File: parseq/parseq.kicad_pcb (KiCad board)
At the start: 2 copper layers, 47.5 x 55 mm, 46 parts, among them J1 Conn_01x01, J2 Conn_01x01, J3 Conn_01x01, J4 Conn_01x01, U1 Opamp_Quad, U2 Opamp_Dual

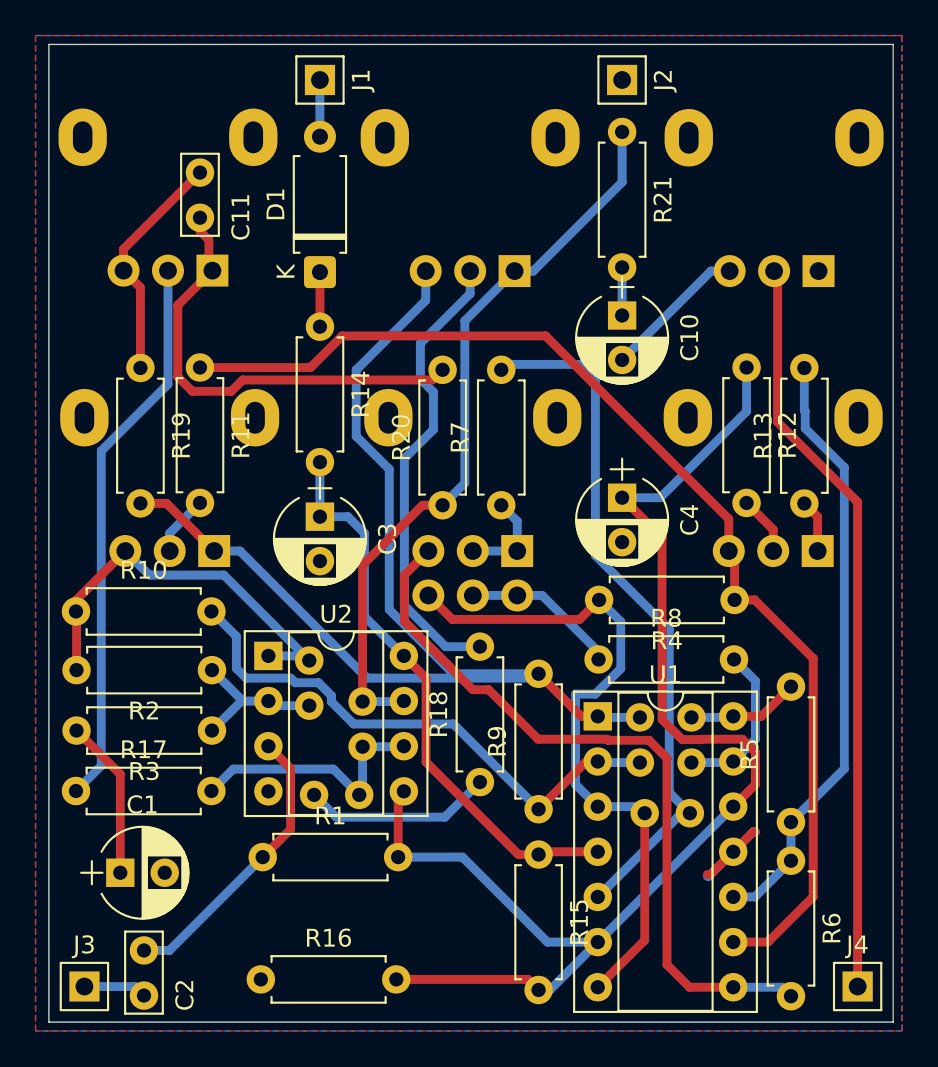
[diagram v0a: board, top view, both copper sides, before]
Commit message: update board
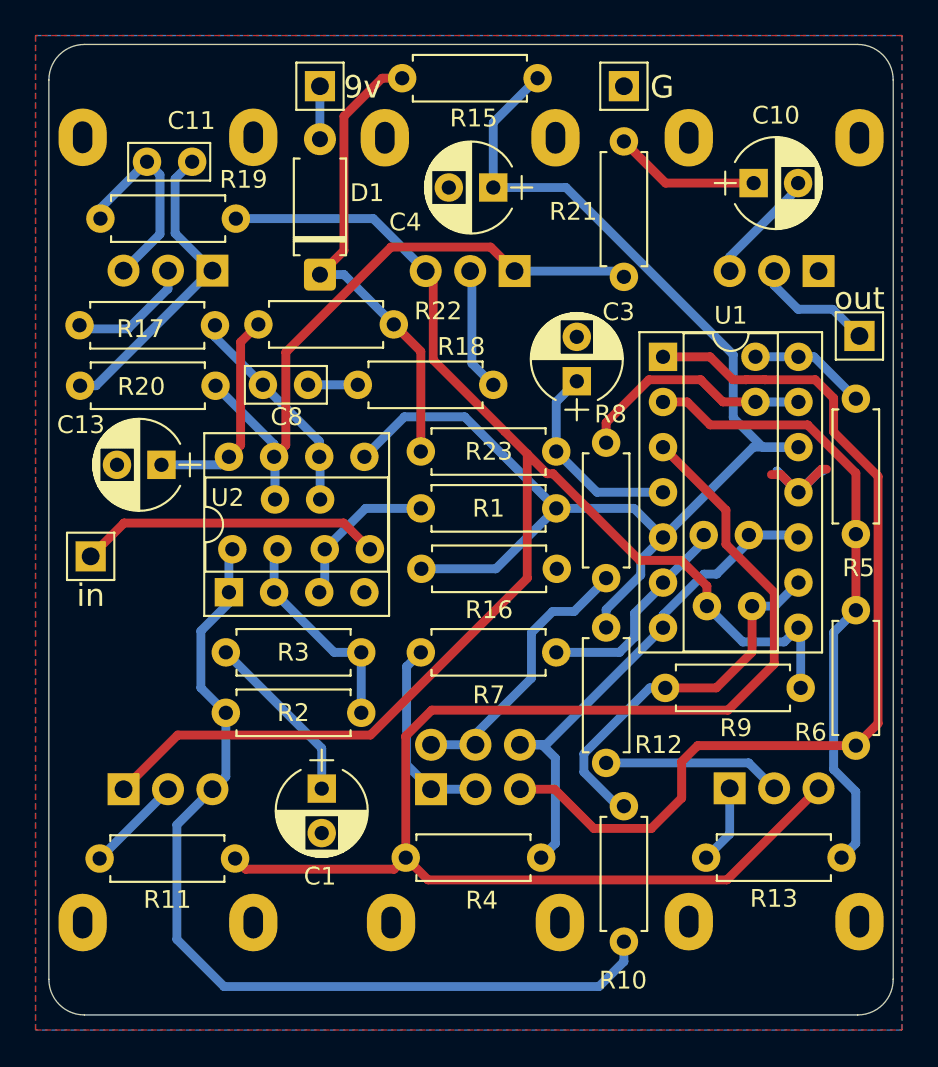
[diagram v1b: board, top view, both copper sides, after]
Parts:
- removed R14: 100, 1_trevortjes_lib:R_1x4
- added C13: 100u, 1_trevortjes_lib:CP_ELCO_1x2_S, F.Cu at (141.6, 84.7)
- added R22: 100, 1_trevortjes_lib:R_1x4, F.Cu at (154.7, 76.8)
- added R23: 100, 1_trevortjes_lib:R_1x4, F.Cu at (156.2, 83.9)
- C2: moved to B.Cu
- C8: moved to F.Cu
- moved R15 44.3 mm to (155.1, 62.9), turned to 0 degrees
- moved J4 36.6 mm to (180.8, 77.4)
- moved R10 36.0 mm to (167.6, 111.5), turned to 90 degrees
- moved R16 28.5 mm to (163.8, 90.5), turned to 180 degrees
- moved R11 27.7 mm to (145.7, 106.8), turned to 180 degrees
- moved R17 26.2 mm to (137.0, 76.8)
- moved C2 24.8 mm to (150.8, 89.4), turned to 0 degrees
- moved J3 24.2 mm to (137.6, 89.8), turned to 180 degrees
- moved R4 23.5 mm to (155.3, 106.8), turned to 0 degrees
- moved R18 23.4 mm to (152.6, 80.2), turned to 0 degrees
- moved C8 23.1 mm to (149.8, 80.2), turned to 180 degrees
- moved R1 21.5 mm to (156.2, 87.1)
- moved R13 20.7 mm to (172.2, 106.8), turned to 0 degrees
- moved C6 20.6 mm to (175.0, 78.6)
- moved U1 20.6 mm to (169.8, 78.6)
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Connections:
- C5 pad 1: Net-(U1A-+) -> Net-(U1C-+)
- C5 pad 2: Net-(U1B-+) -> Net-(U1B--)
- C7 pad 2: Net-(U1A--) -> Net-(U1C--)
- R10 pad 2: Net-(U1A--) -> Net-(U1C--)
- R11 pad 1: Net-(U1C--) -> Net-(U1A-+)
- R13 pad 2: Net-(U1C-+) -> Net-(U1A--)
- R15 pad 1: Net-(U1E-V+) -> Net-(D1-K)
- R4 pad 1: Net-(U1C--) -> Net-(U1A-+)
- R4 pad 2: Net-(U1A-+) -> Net-(U1C-+)
- R5 pad 1: Net-(U1C-+) -> Net-(U1A--)
- R6 pad 1: Net-(U1C-+) -> Net-(U1A--)
- R7 pad 2: Net-(U1B-+) -> Net-(U1B--)
- R9 pad 1: Net-(U1A--) -> Net-(U1C--)
- RV1 pad 6: Net-(U1A-+) -> Net-(U1C-+)
- RV3 pad 3: Net-(U1C--) -> Net-(U1A-+)
- U1 pad 1: Net-(C7-Pad1) -> Net-(RV1A-6)
- U1 pad 5: Net-(U1B-+) -> /vref
- U1 pad 6: /vref -> Net-(U1B--)
- U1 pad 7: Net-(U1A-+) -> Net-(U1C-+)
- U1 pad 8: Net-(RV1A-6) -> Net-(C7-Pad1)
- U2 pad 8: Net-(U1E-V+) -> Net-(U2C-V+)
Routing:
- net Net-(U1C--): track 64.2 -> 21.7 mm
- net Net-(U1A-+): track 38.7 -> 80.0 mm
- net Net-(U1B-+): track 39.6 -> 0.00 mm
- net Net-(J4-Pin_1): track 42.2 -> 6.78 mm
- net Net-(C12-Pad1): track 23.2 -> 52.3 mm
- net Net-(R17-Pad1): track 31.4 -> 7.01 mm
- net Net-(D1-K): track 3.07 -> 26.7 mm
- net Net-(U1E-V+): track 32.1 -> 11.4 mm
- net Net-(R18-Pad2): track 26.2 -> 6.94 mm
- net Net-(C7-Pad1): track 64.9 -> 83.2 mm
- net Net-(J3-Pin_1): track 3.56 -> 17.1 mm
- net Net-(RV1A-6): track 41.8 -> 54.6 mm
- net Net-(U2C-V+): track 0.00 -> 12.1 mm
- net Net-(U1B--): track 0.00 -> 12.1 mm
- net Net-(C11-Pad2): track 25.8 -> 17.5 mm
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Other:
- board size 47.5 x 55 mm -> 47.5 x 54.6 mm
- board text added: "125b between screws (in long dimension)"
